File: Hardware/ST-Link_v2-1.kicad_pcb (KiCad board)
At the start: 2 copper layers, 31.1 x 14.4 mm, 35 parts, among them J1 Conn_01x06, P1 USB_C_Plug_USB2.0, U1 STM32F103CBTx, U2 LP5907MFX-3.3, Y1 Crystal_Small

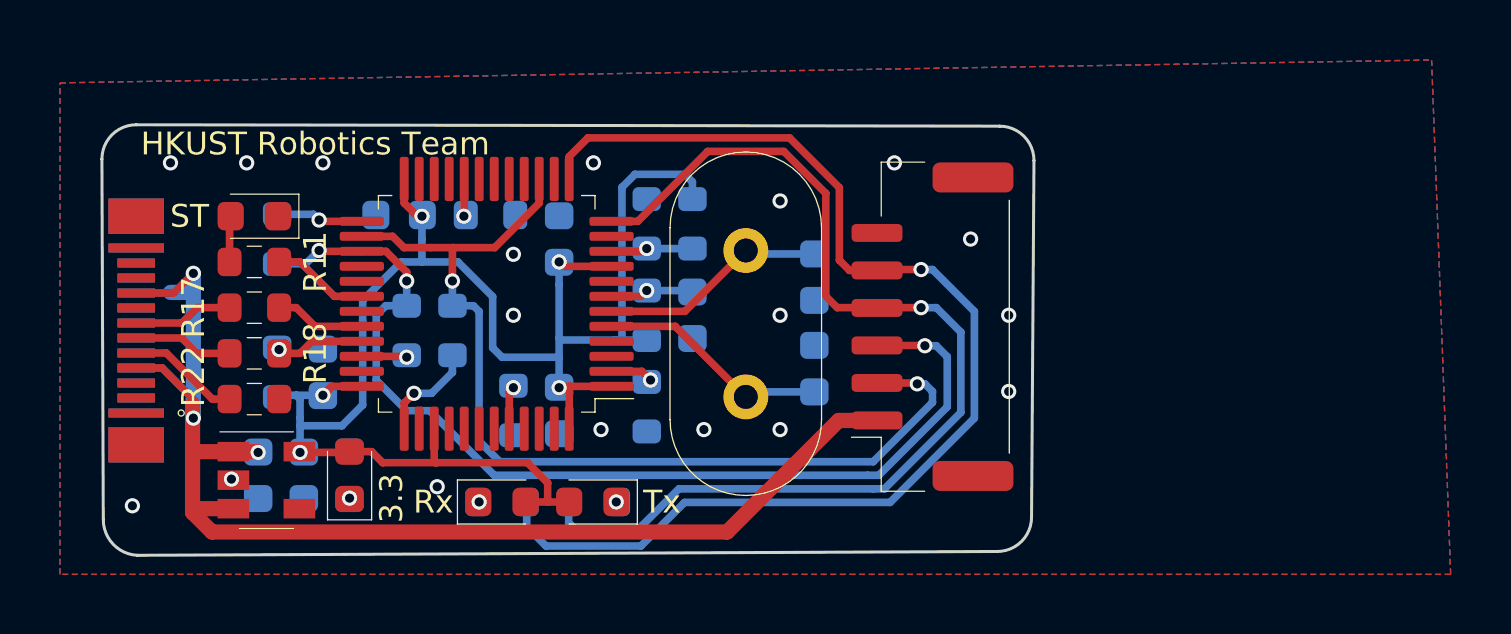
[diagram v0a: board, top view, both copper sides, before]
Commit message: readme
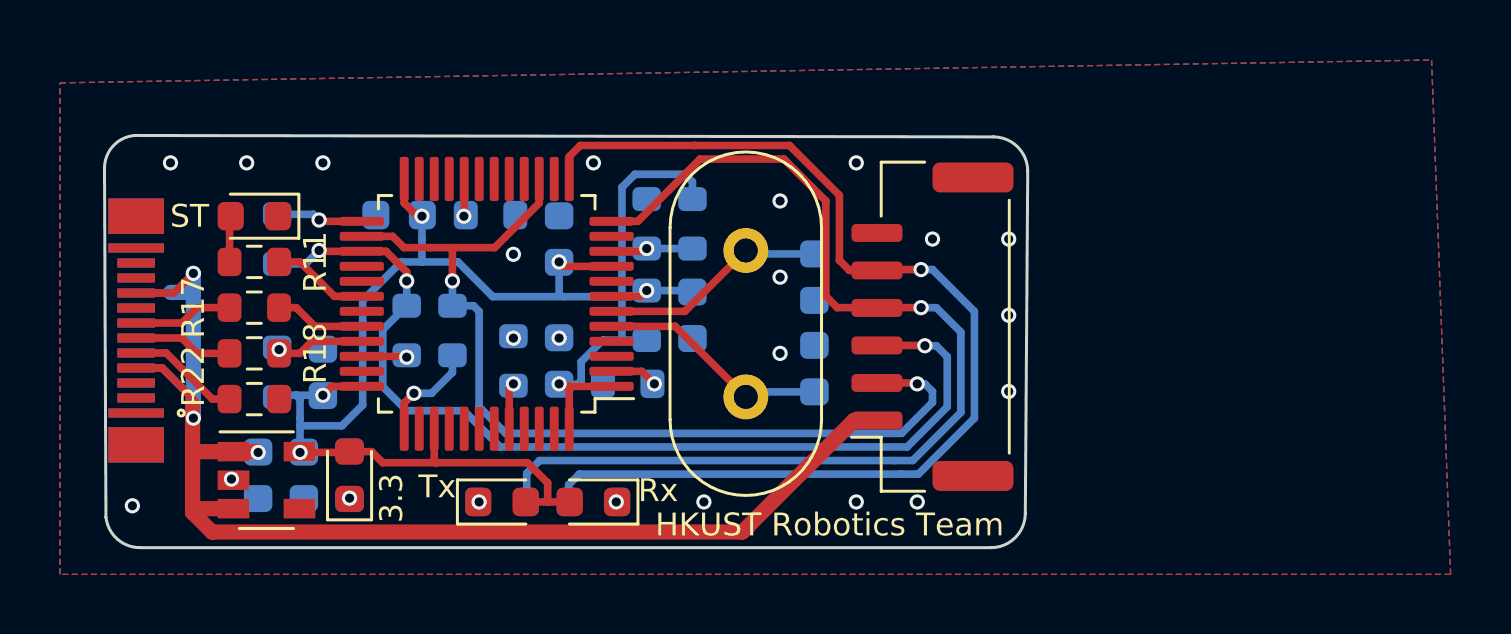
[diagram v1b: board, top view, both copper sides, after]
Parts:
- moved R4 3.05 mm to (153.3, 112.9), turned to 180 degrees
- moved R5 3.05 mm to (156.3, 112.9), turned to 0 degrees
- moved Rx 3.05 mm to (156.3, 112.9), turned to 180 degrees
- moved Tx 3.03 mm to (153.3, 112.9), turned to 0 degrees
- moved C5 1.65 mm to (155.2, 108.2), turned to 90 degrees
- moved R6 1.65 mm to (153.7, 108.2), turned to 90 degrees
- moved R9 0.99 mm to (157.5, 109.0), turned to 180 degrees
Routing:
- net /RXD: track 39.7 -> 36.6 mm
- net +3V3: track 55.6 -> 53.7 mm
- net /JTCK: track 33.3 -> 31.8 mm
- net /JTMS: track 34.7 -> 33.3 mm
- net GND: vias 18 -> 20
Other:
- board size 31.1 x 14.4 mm -> 30.8 x 13.7 mm
